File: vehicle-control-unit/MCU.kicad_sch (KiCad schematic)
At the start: 97 parts, among them J4 FTSH-107-01-F-DV-K-P-TR, Q10 AO3400A, Q6 AO3400A, Q7 AO3400A, Q8 AO3400A, Q9 AO3400A, SW4 PV1H240BB, SW5 Y97KT23B5NAFP, U17 PST360G2-2AA-C0123-ERA040-05K, U18 PST360G2-2AA-C0123-ERA040-05K, U19 PST360G2-2AA-C0123-ERA040-05K, U21 ISO1044BD, U22 ISO1044BD, U24 MCP6004, U25 104990302, U26 STLINK-V3MODS, U27 STM32F446RETx, Y1 ECS-240-8-37B-CKY-TR

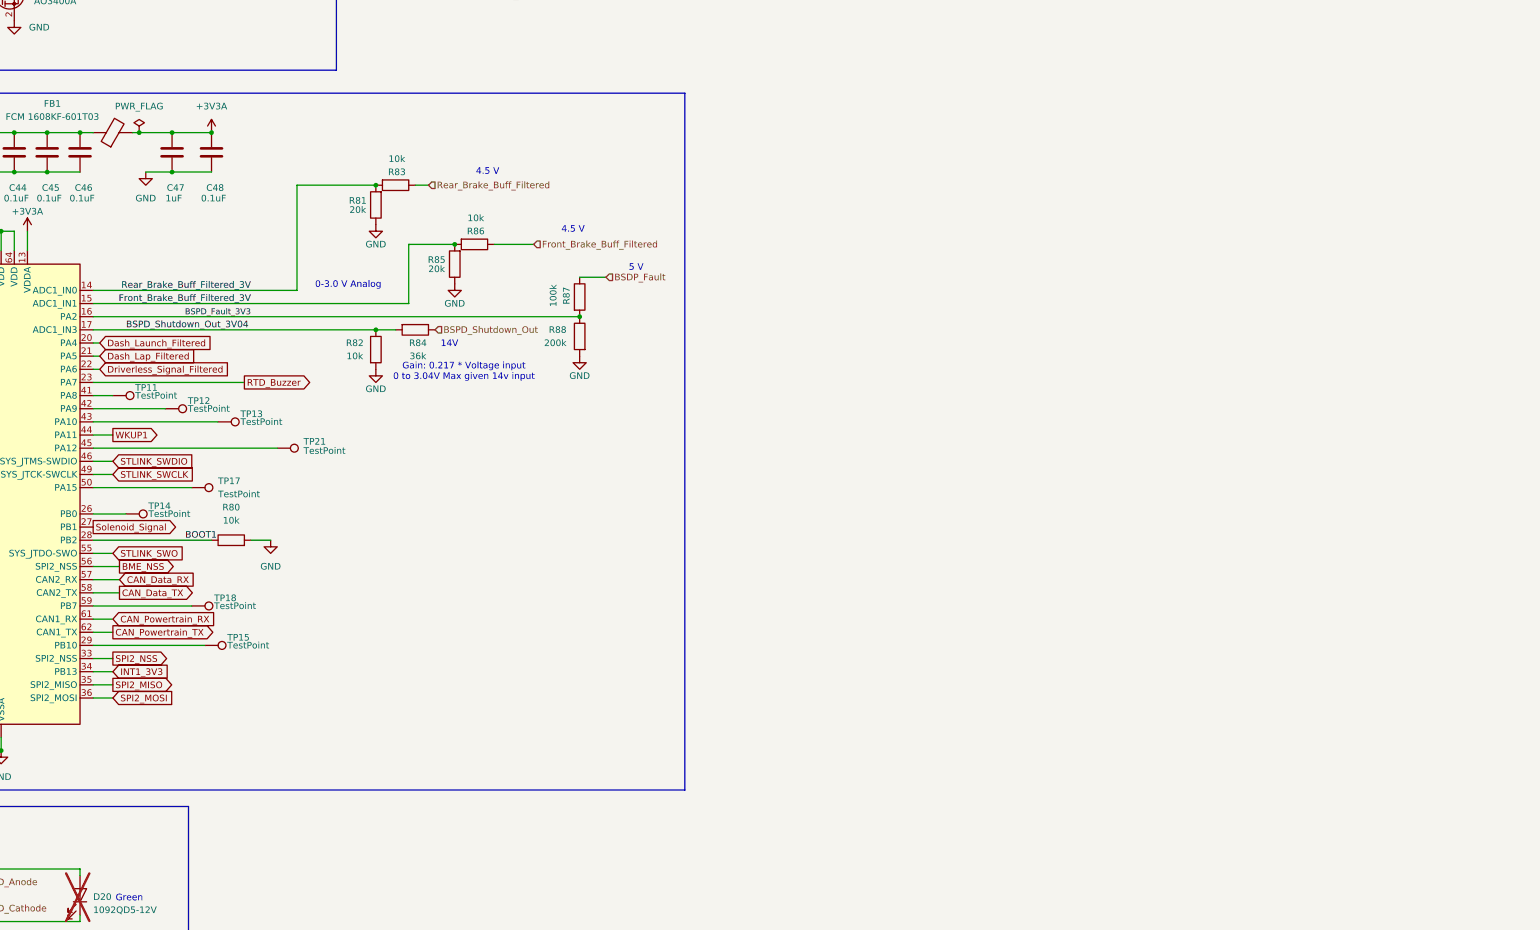
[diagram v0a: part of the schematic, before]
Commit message: vcu changes progess
-new mcu added and pairing progess
-grounding clips added
-changed schematic symbols to fs_components library
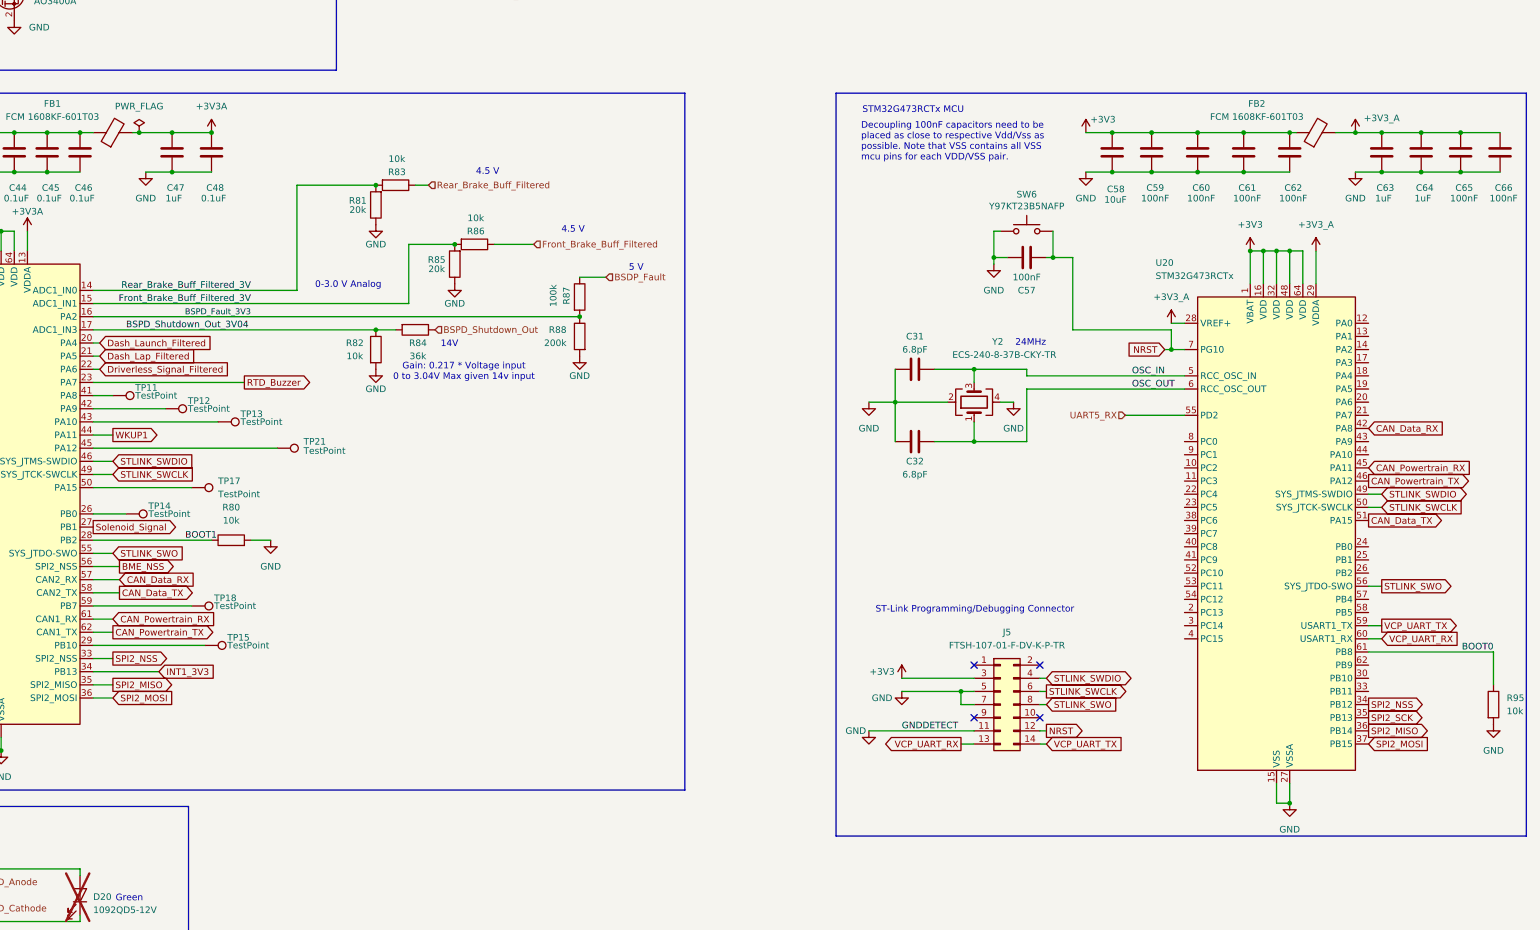
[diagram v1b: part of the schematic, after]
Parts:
- added C31, C32: 6.8pF, Capacitor_SMD:C_0603_1608Metric_Pad1.08x0.95mm_HandSolder, symbol Device:C
- added C57, C59, C60, C61, C62, C65, C66: 100nF, Capacitor_SMD:C_0603_1608Metric_Pad1.08x0.95mm_HandSolder, symbol Device:C
- added C58: 10uF, Capacitor_SMD:C_0603_1608Metric_Pad1.08x0.95mm_HandSolder, symbol Device:C
- added C63, C64: 1uF, Capacitor_SMD:C_0603_1608Metric_Pad1.08x0.95mm_HandSolder, symbol Device:C
- added FB2: FCM 1608KF-601T03, Inductor_SMD:L_0603_1608Metric_Pad1.05x0.95mm_HandSolder, symbol Device:FerriteBead
- added J5: FTSH-107-01-F-DV-K-P-TR, Connector_PinHeader_1.27mm:PinHeader_2x07_P1.27mm_Vertical_SMD, symbol Connector_Generic:Conn_02x07_Odd_Even
- added R95: 10k, Resistor_SMD:R_0603_1608Metric_Pad0.98x0.95mm_HandSolder, symbol Device:R
- added SW6: Y97KT23B5NAFP, Button_Switch_SMD:SW_SPST_PTS647_Sx38, symbol Switch:SW_Push
- added U20: STM32G473RCTx, Package_QFP:LQFP-64_10x10mm_P0.5mm, symbol MCU_ST_STM32G4:STM32G473RCTx
- added Y2: ECS-240-8-37B-CKY-TR, Crystal:Crystal_SMD_2016-4Pin_2.0x1.6mm, symbol Device:Crystal_GND24
- U21, U22: footprint FS_4_Global_Footprint_Library:SOIC-8_ISO1044BD -> formula_slug_footprint_library:SOIC-8_ISO1044BD
- U26: footprint FS_4_Global_Footprint_Library:MODULE_STLINK-V3MODS -> formula_slug_footprint_library:MODULE_STLINK-V3MODS
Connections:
- net +3V3: now also C58.2, C59.1, C60.1, C61.1, C62.1, FB2.1, J5.3 (Pin_3), U20.1 (VBAT), U20.16 (VDD), U20.32 (VDD), U20.48 (VDD), U20.64 (VDD)
- net BOOT0: now also R95.1, U20.61 (PB8)
- net CAN_Data_RX: now also U20.42 (PA8)
- net CAN_Data_TX: now also U20.51 (PA15)
- net CAN_Powertrain_RX: now also U20.45 (PA11)
- net CAN_Powertrain_TX: now also U20.46 (PA12)
- net GND: now also C31.2, C32.2, C57.1, C58.1, C59.2, C60.2, C61.2, C62.2, C63.2, C64.2, C65.2, C66.2, J5.11 (Pin_11), J5.5 (Pin_5), J5.7 (Pin_7), R95.2, SW6.1, U20.15 (VSS), U20.27 (VSSA), U20.31 (VSS), U20.47 (VSS), U20.63 (VSS), Y2.2, Y2.4
- net NRST: now also C57.2, J5.12 (Pin_12), SW6.2, U20.7 (PG10)
- net OSC_IN: now also C31.1, U20.5 (PF0), Y2.3
- net OSC_OUT: now also C32.1, U20.6 (PF1), Y2.1
- net SPI2_MISO: now also U20.36 (PB14)
- net SPI2_MOSI: now also U20.37 (PB15)
- net SPI2_NSS: now also U20.34 (PB12)
- net SPI2_SCK: now also U20.35 (PB13)
- net STLINK_SWCLK: now also J5.6 (Pin_6), U20.50 (PA14)
- net STLINK_SWDIO: now also J5.4 (Pin_4), U20.49 (PA13)
- net STLINK_SWO: now also J5.8 (Pin_8), U20.56 (PB3)
- net UART5_RX: now also U20.55 (PD2)
- new net +3V3_A: C63.1, C64.1, C65.1, C66.1, FB2.2, U20.28 (VREF+), U20.29 (VDDA)
- new net VCP_UART_RX: J5.13 (Pin_13), U20.60 (PB7)
- new net VCP_UART_TX: J5.14 (Pin_14), U20.59 (PB6)
- no-connect marks 32 -> 36
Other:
- note added: "24MHz"
- note added: "Decoupling 100nF capacitors need to be placed as close to respective Vdd/Vss as possible. Note that VSS contains all VSS mcu pins for each VDD/VSS pair."
- note added: "STM32G473RCTx MCU"

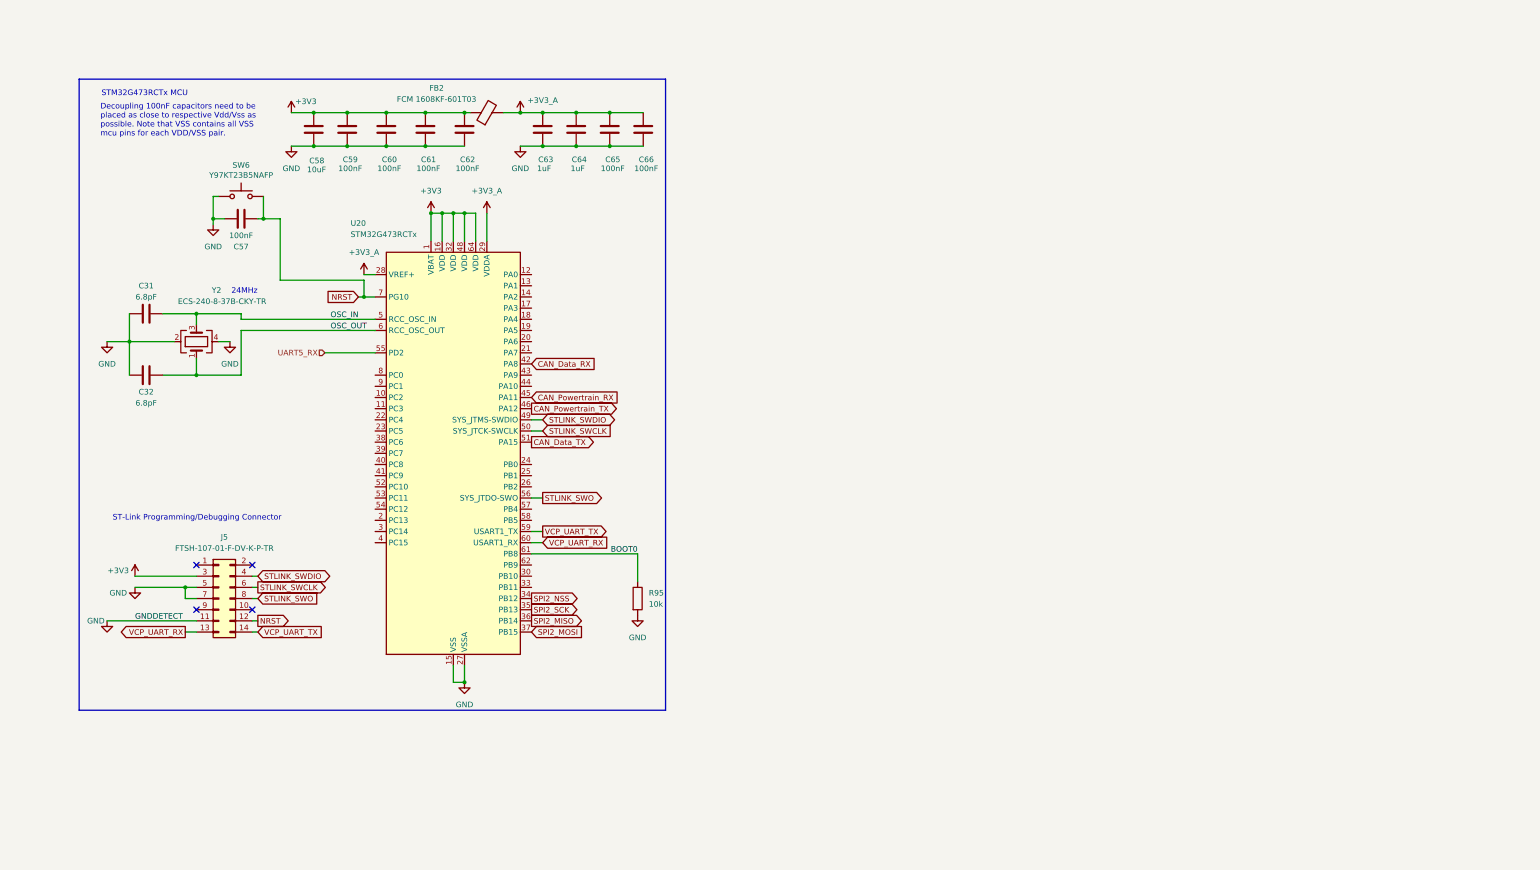
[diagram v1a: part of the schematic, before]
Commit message: progress on new mcu, ground clip added
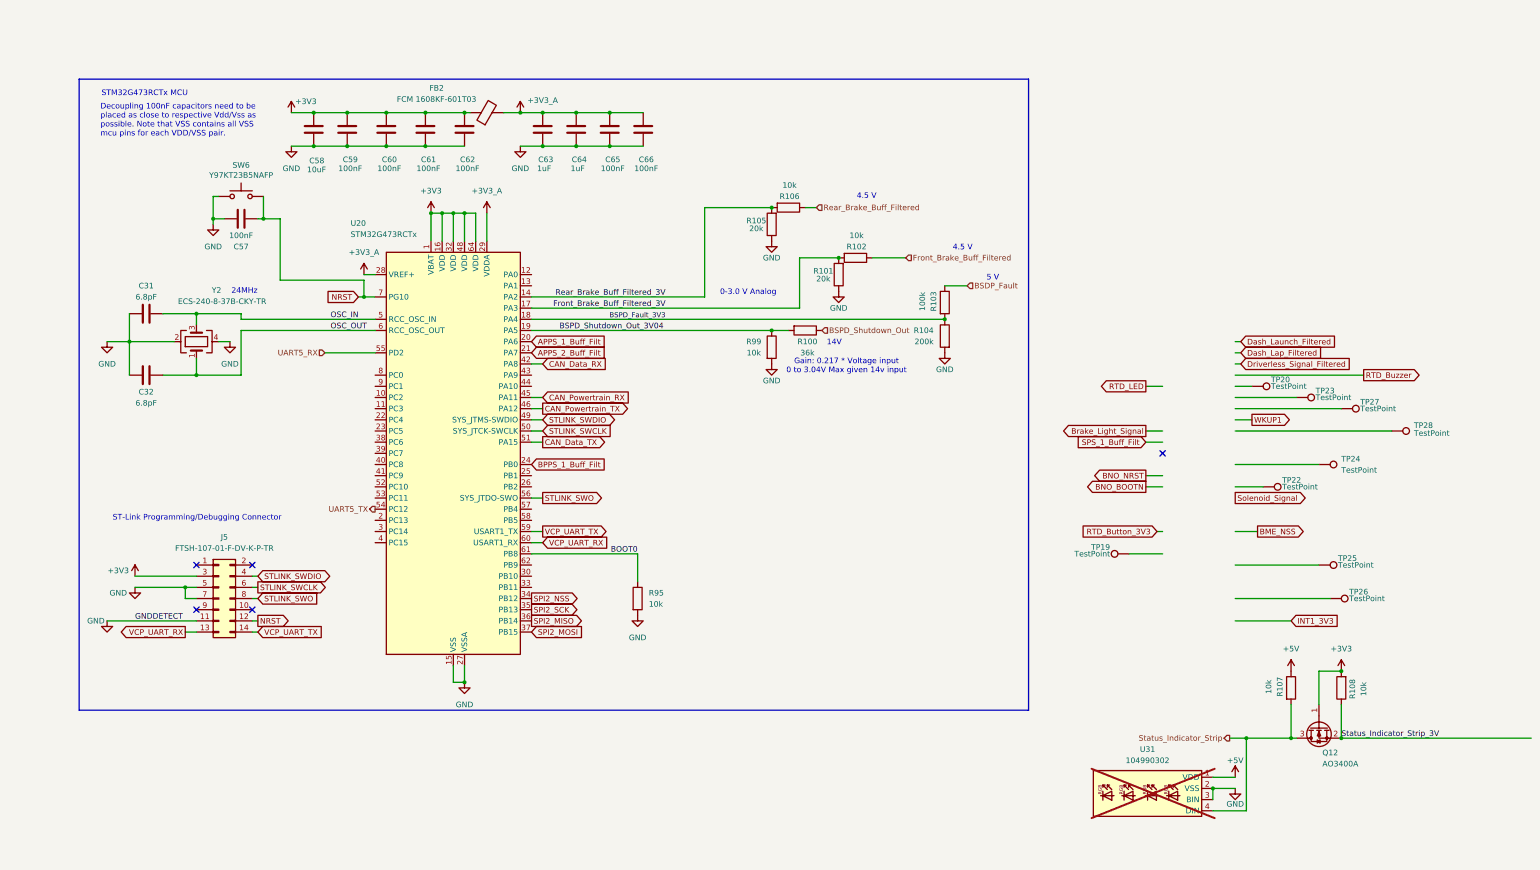
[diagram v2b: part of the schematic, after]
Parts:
- added Q12: AO3400A, Package_TO_SOT_SMD:SOT-23, symbol Transistor_FET:AO3400A
- added R100: 36k, Resistor_SMD:R_0603_1608Metric_Pad0.98x0.95mm_HandSolder, symbol Device:R
- added R101, R105: 20k, Resistor_SMD:R_0603_1608Metric_Pad0.98x0.95mm_HandSolder, symbol Device:R
- added R102, R106, R107, R108, R99: 10k, Resistor_SMD:R_0603_1608Metric_Pad0.98x0.95mm_HandSolder, symbol Device:R
- added R103: 100k, Resistor_SMD:R_0603_1608Metric_Pad0.98x0.95mm_HandSolder, symbol Device:R
- added R104: 200k, Resistor_SMD:R_0603_1608Metric_Pad0.98x0.95mm_HandSolder, symbol Device:R
- added TP19, TP20, TP22, TP23, TP24, TP25, TP26, TP27, TP28: TestPoint, TestPoint:TestPoint_Pad_D1.0mm, symbol Connector:TestPoint
- added U31: 104990302, symbol FS_4_Global_Symbol_Library:WS2813B
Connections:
- net +3V3: now also Q12.1 (G), R108.2
- net +5V: now also R107.1, U31.1 (VDD)
- net APPS_1_Buff_Filt: now also U20.20 (PA6)
- net APPS_2_Buff_Filt: now also U20.21 (PA7)
- net BPPS_1_Buff_Filt: now also U20.24 (PB0)
- net BSDP_Fault: now also R103.1
- net BSPD_Fault_3V3: now also U20.18 (PA4), R103.2, R104.1
- net BSPD_Shutdown_Out: now also R100.1
- net BSPD_Shutdown_Out_3V04: now also U20.19 (PA5), R100.2, R99.1
- net Front_Brake_Buff_Filtered: now also R102.1
- net Front_Brake_Buff_Filtered_3V: now also U20.17 (PA3), R101.2, R102.2
- net GND: now also R101.1, R104.2, R105.1, R99.2, U31.2 (VSS), U31.3 (BIN)
- net Rear_Brake_Buff_Filtered: now also R106.1
- net Rear_Brake_Buff_Filtered_3V: now also U20.14 (PA2), R105.2, R106.2
- net Status_Indicator_Strip: now also Q12.3 (D), R107.2, U31.4 (DIN)
- net Status_Indicator_Strip_3V: now also Q12.2 (S), R108.1
- net UART5_TX: now also U20.54 (PC12)
- no-connect marks 36 -> 37

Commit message: Schematic changes
-STM32G473 mcu added
-sampling of shutdown nets
-test points to important nets
-debug led
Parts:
- removed C37, C38: 6.8pF, Capacitor_SMD:C_0603_1608Metric_Pad1.08x0.95mm_HandSolder, symbol Device:C
- removed C40, C43, C44, C45, C46, C48: 0.1uF, Capacitor_SMD:C_0603_1608Metric_Pad1.08x0.95mm_HandSolder, symbol Device:C
- removed C41: 4.7uF, Capacitor_SMD:C_0603_1608Metric_Pad1.08x0.95mm_HandSolder, symbol Device:C
- removed C42: 10uF, Capacitor_SMD:C_0603_1608Metric_Pad1.08x0.95mm_HandSolder, symbol Device:C
- removed C47: 1uF, Capacitor_SMD:C_0603_1608Metric_Pad1.08x0.95mm_HandSolder, symbol Device:C
- removed FB1: FCM 1608KF-601T03, Inductor_SMD:L_0603_1608Metric_Pad1.05x0.95mm_HandSolder, symbol Device:FerriteBead
- removed J4: FTSH-107-01-F-DV-K-P-TR, Connector_PinHeader_1.27mm:PinHeader_2x07_P1.27mm_Vertical_SMD, symbol Connector_Generic:Conn_02x07_Odd_Even
- removed Q6: AO3400A, Package_TO_SOT_SMD:SOT-23, symbol Transistor_FET:AO3400A
- removed R71, R72, R73, R80, R82, R83, R86: 10k, Resistor_SMD:R_0603_1608Metric_Pad0.98x0.95mm_HandSolder, symbol Device:R
- removed R81, R85: 20k, Resistor_SMD:R_0603_1608Metric_Pad0.98x0.95mm_HandSolder, symbol Device:R
- removed R84: 36k, Resistor_SMD:R_0603_1608Metric_Pad0.98x0.95mm_HandSolder, symbol Device:R
- removed R87: 100k, Resistor_SMD:R_0603_1608Metric_Pad0.98x0.95mm_HandSolder, symbol Device:R
- removed R88: 200k, Resistor_SMD:R_0603_1608Metric_Pad0.98x0.95mm_HandSolder, symbol Device:R
- removed SW5: Y97KT23B5NAFP, Button_Switch_SMD:SW_SPST_PTS647_Sx38, symbol Switch:SW_Push
- removed TP11, TP12, TP13, TP14, TP15, TP16, TP17, TP18, TP20, TP21, TP22, TP25, TP26, TP27, TP28: TestPoint, TestPoint:TestPoint_Pad_D1.0mm, symbol Connector:TestPoint
- removed U25: 104990302, symbol FS_4_Global_Symbol_Library:WS2813B
- removed U27: STM32F446RETx, Package_QFP:LQFP-64_10x10mm_P0.5mm, symbol MCU_ST_STM32F4:STM32F446RETx
- removed Y1: ECS-240-8-37B-CKY-TR, Crystal:Crystal_SMD_2016-4Pin_2.0x1.6mm, symbol Device:Crystal_GND24
- added D23: LTST-S270KRKT, LED_SMD:LED_0603_1608Metric_Pad1.05x0.95mm_HandSolder, symbol Device:LED
- added R96: 300, Resistor_SMD:R_0603_1608Metric_Pad0.98x0.95mm_HandSolder, symbol Device:R
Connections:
- net APPS_1_Buff_Filt: now also U20.9 (PC1); no longer U20.20 (PA6)
- net APPS_2_Buff_Filt: now also U20.10 (PC2); no longer U20.21 (PA7)
- net BME_NSS: now also U20.30 (PB10)
- net BNO_BOOTN: now also U20.40 (PC8)
- net BNO_NRST: now also U20.39 (PC7)
- net BOOT0: now also TP23.1
- net BPPS_1_Buff_Filt: now also U20.11 (PC3); no longer U20.24 (PB0)
- net BSPD_Fault_3V3: now also U20.14 (PA2); no longer U20.18 (PA4)
- net BSPD_Shutdown_Out: now also U20.43 (PA9)
- net BSPD_Shutdown_Out_3V04: now also U20.17 (PA3); no longer U20.19 (PA5)
- net Brake_Light_Signal: now also U20.38 (PC6)
- net Dash_Lap_Filtered: now also U20.58 (PB5)
- net Dash_Launch_Filtered: now also U20.57 (PB4)
- net Driverless_Signal_Filtered: now also U20.4 (PC15)
- net Front_Brake_Buff_Filtered_3V: now also U20.13 (PA1); no longer U20.17 (PA3)
- net GND: now also D23.1 (K)
- net INT1_3V3: now also U20.62 (PB9)
- net RTD_Button_3V3: now also U20.2 (PC13)
- net RTD_Buzzer: now also U20.23 (PC5)
- net RTD_LED: now also U20.8 (PC0)
- net Rear_Brake_Buff_Filtered_3V: now also U20.12 (PA0); no longer U20.14 (PA2)
- net SPS_1_Buff_Filt: now also U20.41 (PC9)
- net STLINK_SWO: no longer U20.56 (PB3)
- net Solenoid_Signal: now also U20.52 (PC10)
- net Status_Indicator_Strip_3V: now also U20.3 (PC14)
- net WKUP1: now also U20.44 (PA10)
- net Current_Sensor_Fault: now reaches U20.22 (PC4)
- net Rear_Brake_Fault: now reaches U20.25 (PB1)
- net Hard_Braking_High_Current: now reaches U20.26 (PB2)
- net BSPD_Fault: now reaches U20.33 (PB11)
- net at U20.53 (PC11): now also TP19.1
- net at TP24.1: now also U20.56 (PB3), R96.2
- new net: D23.2 (A), R96.1
- new net BOTS_Shutdown: U20.20 (PA6)
- new net E_Stop_Shutdown: U20.21 (PA7)
- new net Front_Brake_Fault: U20.24 (PB0)
- new net Inertia_Shutdown: U20.18 (PA4)
- new net Shutdown_In: U20.19 (PA5)
- no-connect marks 37 -> 32
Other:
- note added: "RED LED"
- note removed: "Microcontroller"
